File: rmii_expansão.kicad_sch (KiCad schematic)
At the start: 6 parts, among them CN3 100nf, J19 ETH

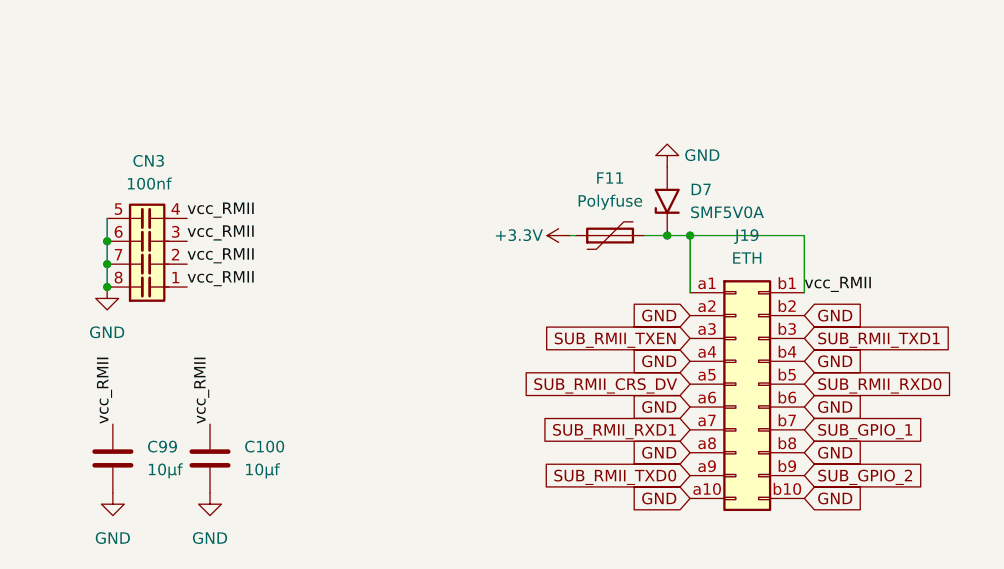
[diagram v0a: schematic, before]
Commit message: 29082026/I
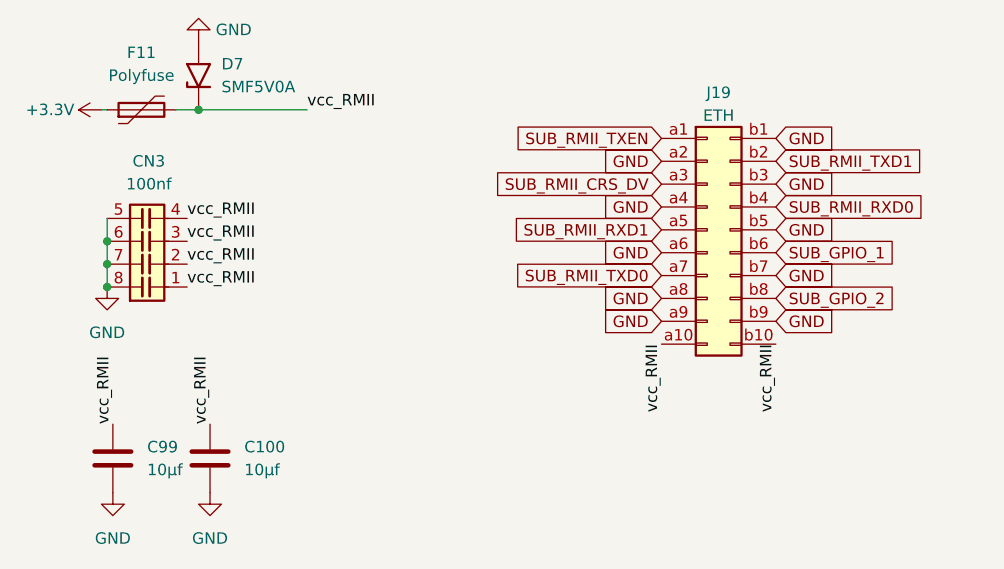
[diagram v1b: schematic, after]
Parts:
- CN3: jlc_pcb: C346191 -> C307348; mouser: (none) -> 187-CL10B104KB8WPNC; mpn CA0612MRX7R7BB104 -> CL10B104KB8WPNC
- J19: footprint (none) -> Connector_PinHeader_2.54mm:PinHeader_2x10_P2.54mm_Horizontal; Descrição (none) -> o da lcsc e da mouser sâo diferente; jlc_pcb: (none) -> C53207373; mouser: (none) -> 649-68021-120HLF; mpn (none) -> PZ-2.54-2*10-8.5-WZ
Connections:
- net GND: now also J19.a9 (Pin_a9), J19.b1 (Pin_b1), J19.b3 (Pin_b3), J19.b5 (Pin_b5), J19.b7 (Pin_b7), J19.b9 (Pin_b9); no longer J19.a10 (Pin_a10), J19.b10 (Pin_b10), J19.b2 (Pin_b2), J19.b4 (Pin_b4), J19.b6 (Pin_b6), J19.b8 (Pin_b8)
- net SUB_GPIO_1: now also J19.b6 (Pin_b6); no longer J19.b7 (Pin_b7)
- net SUB_GPIO_2: now also J19.b8 (Pin_b8); no longer J19.b9 (Pin_b9)
- net SUB_RMII_CRS_DV: now also J19.a3 (Pin_a3); no longer J19.a5 (Pin_a5)
- net SUB_RMII_RXD0: now also J19.b4 (Pin_b4); no longer J19.b5 (Pin_b5)
- net SUB_RMII_RXD1: now also J19.a5 (Pin_a5); no longer J19.a7 (Pin_a7)
- net SUB_RMII_TXD0: now also J19.a7 (Pin_a7); no longer J19.a9 (Pin_a9)
- net SUB_RMII_TXD1: now also J19.b2 (Pin_b2); no longer J19.b3 (Pin_b3)
- net SUB_RMII_TXEN: now also J19.a1 (Pin_a1); no longer J19.a3 (Pin_a3)
- net vcc_RMII: now also J19.a10 (Pin_a10), J19.b10 (Pin_b10); no longer J19.a1 (Pin_a1), J19.b1 (Pin_b1)
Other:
- company: (none) -> ---
- title: (none) -> expansão com ethernet
- moved on the sheet: D7, F11, J19
